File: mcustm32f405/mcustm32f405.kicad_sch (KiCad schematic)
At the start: 36 parts, among them J2 STM32WORLD_CONNECTOR_1, J3 STM32WORLD_CONNECTOR_2, J4 STM32WORLD_BOARD, SW1 TS-1088R-02526, SW2 TS-1088R-02526, U1 AMS1117-3.3, U2 SRV05-4, U3 STM32F405RGTx, Y1 X_16MHZ

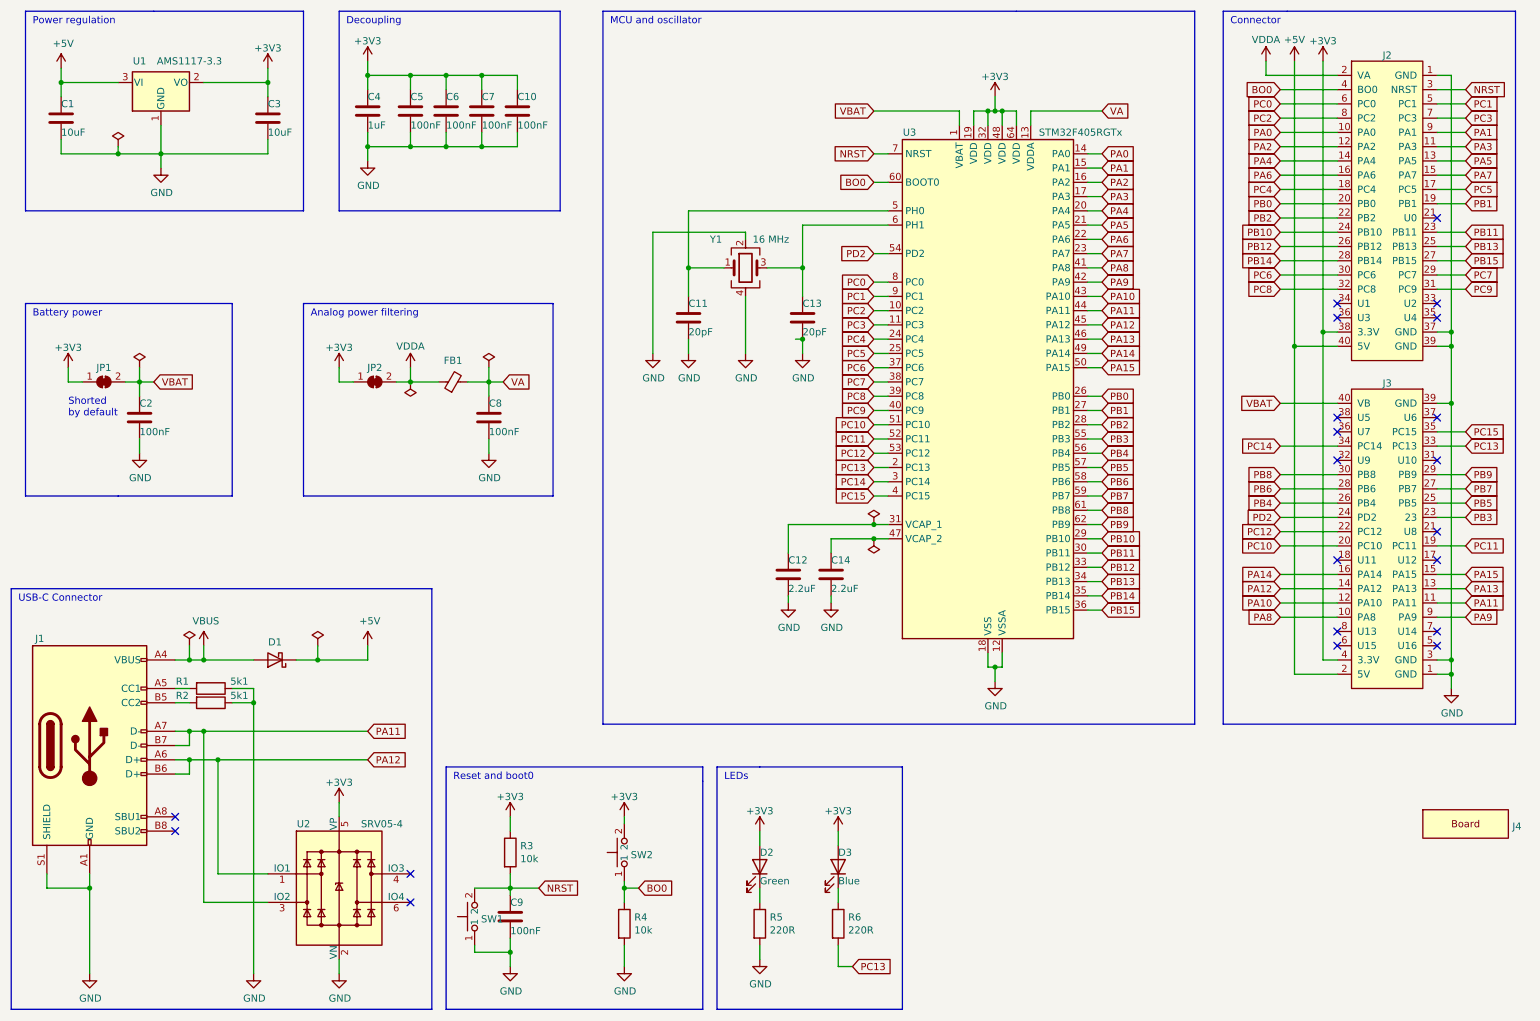
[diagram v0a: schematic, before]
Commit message: Hmmm
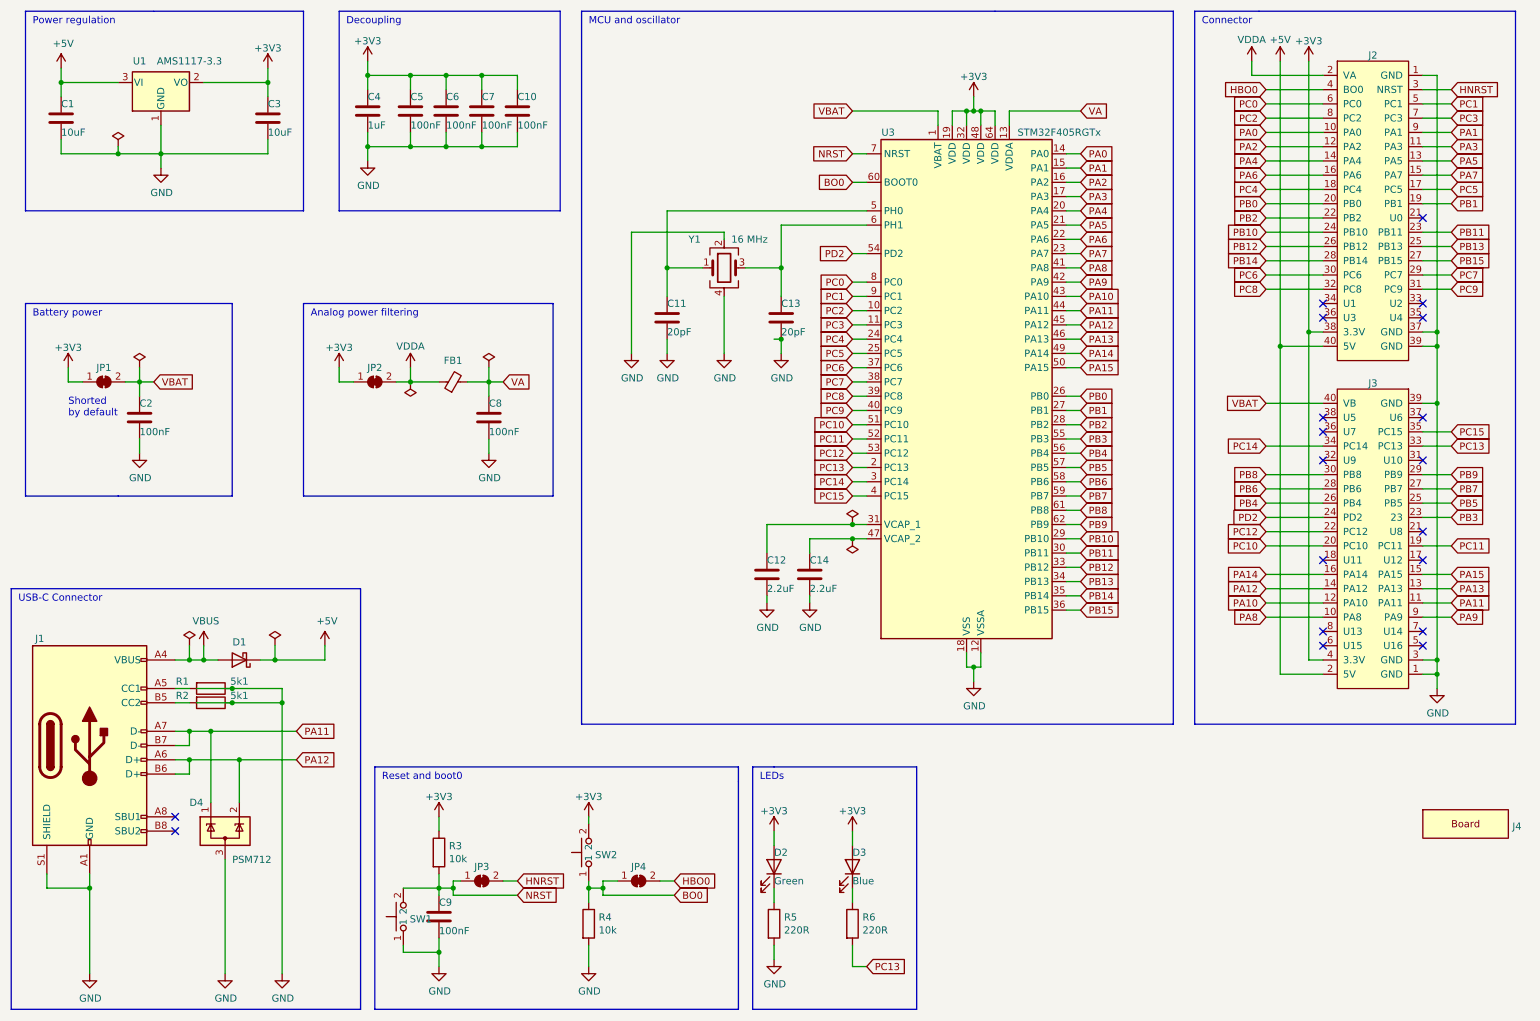
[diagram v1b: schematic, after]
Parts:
- removed U2: SRV05-4, Package_TO_SOT_SMD:SOT-23-6, symbol stm32world:SRV05-4
- added D4: PSM712, Package_TO_SOT_SMD:SOT-23, symbol Power_Protection:SP0502BAHT
- added JP3, JP4: SolderJumper_2_Bridged, Jumper:SolderJumper-2_P1.3mm_Bridged_RoundedPad1.0x1.5mm, symbol stm32world:SolderJumper_2_Bridged
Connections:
- net BO0: now also JP4.1 (A); no longer J2.4 (BO0)
- net GND: now also D4.3 (A)
- net NRST: now also JP3.1 (A); no longer J2.3 (NRST)
- net PA11: now also D4.1 (K)
- net PA12: now also D4.2 (K)
- new net HBO0: J2.4 (BO0), JP4.2 (B)
- new net HNRST: J2.3 (NRST), JP3.2 (B)
- no-connect marks 21 -> 19
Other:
- moved on the sheet: C11, C12, C13, C14, C9, D1, D2, D3, J2, J3, R3, R4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
